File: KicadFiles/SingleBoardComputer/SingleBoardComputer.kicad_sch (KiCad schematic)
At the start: 83 parts, among them J1 USB_C_Receptacle_USB2.0_16P, J2 Conn_01x10_Pin, J3 Conn_01x06_Pin, J4 Conn_01x06_Pin, J5 Conn_01x06_Pin, SW1 SW_DPST_x2_Custom, U1 8468-11B1-RK-TP, U10 AS7C1026B-12JCN, U11 XC9572XL-PC44, U12 SST39SF040-70-4C-PHE, U13 SST39SF040-70-4C-PHE, U2 TLV809EA46DBZR, U3 TPS630701RNMT, U4 FT240XS, U5 LD1117S33TR_SOT223, U6 8444-11B1-RK-TP, U7 4832-6000-CP, U8 4832-6000-CP, U9 MC68000FN, Y1 CXO_DIP8

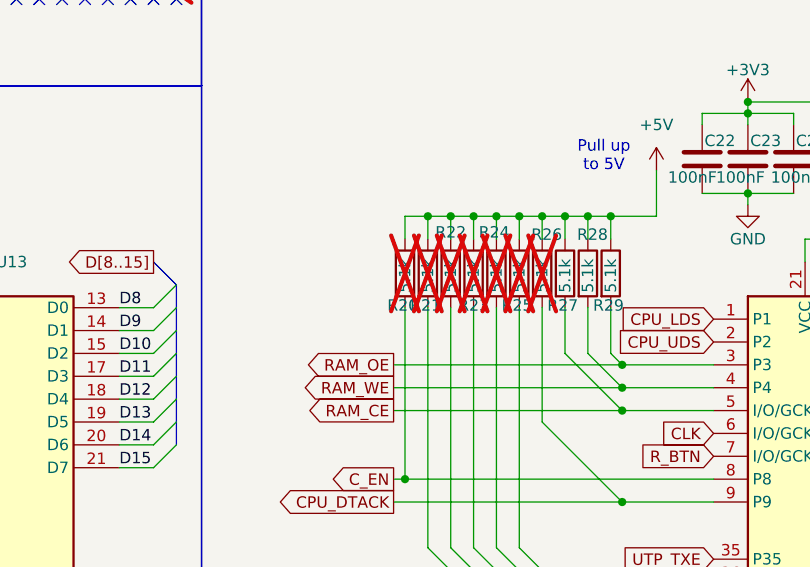
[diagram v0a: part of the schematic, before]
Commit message: PCB done
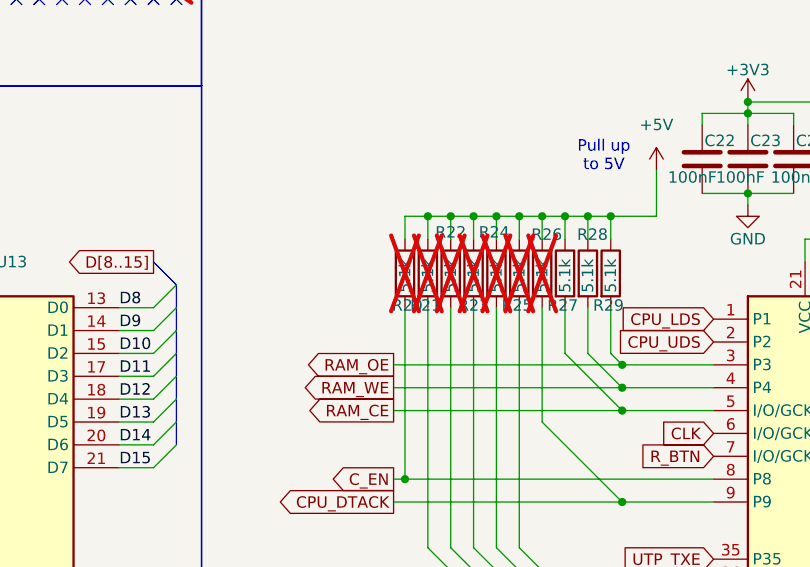
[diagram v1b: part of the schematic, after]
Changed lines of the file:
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@@
 			)
 		)
-		(property "Datasheet" "~"
+		(property "Datasheet" "https://www.digikey.com/en/products/detail/amphenol-cs-commercial-products/G800W302018EU/17069165"
 			(at 262.89 151.13 0)
 			(effects
@@
 			)
 		)
-		(property "Datasheet" "https://www.digikey.com/en/products/detail/adam-tech/PH1-10-UA/9830653?s=N4IgjCBcoGwJxVAYygMwIYBsDOBTANCAPZQDaIALGGABxwDsIAuoQA4AuUIAyuwE4BLAHYBzEAF9CNGohApIGHAWJkQMAMxwaMZm06Qe-YWMkg4ABlnzFeQiUjlNMGAFZdIDl16DREwmHh1KzQsWxUHEHUwODgAJgQWD31DHxN-egtghVDle3IGWJ1EzwNvYz9wLQRoORClO1VLJlNY81iIGuschoiqehoXBL0vI19TAFoZTrqwvJBWl0ZmwnGdach%2BAFdc1SDlkHHYrK2diLd98erkKBOe8ghm8XEgA"
+		(property "Datasheet" "https://www.digikey.com/en/products/detail/amphenol-cs-fci/10129378-910002BLF/7915958"
 			(at 180.34 105.41 0)
 			(effects
@@
 			)
 		)
-		(property "Datasheet" "https://www.digikey.com/en/products/detail/adam-tech/ADT-AMP1251106S4BS165A1/9832042"
+		(property "Datasheet" "https://www.digikey.com/en/products/detail/amphenol-cs-commercial-products/G800W302018EU/17069165"
 			(at 290.83 109.22 0)
 			(effects
@@
 		(lib_id "Device:R")
 		(at 208.28 191.77 0)
+		(mirror y)
 		(unit 1)
 		(exclude_from_sim no)
@@
 		(dnp yes)
 		(property "Reference" "R20"
-			(at 208.026 195.326 0)
+			(at 208.534 195.326 0)
 			(effects
 				(font
@@
 		)
 		(property "Footprint" "Resistor_SMD:R_0805_2012Metric_Pad1.20x1.40mm_HandSolder"
-			(at 206.502 191.77 90)
+			(at 210.058 191.77 90)
 			(effects
 				(font
@@
 			)
 		)
-		(property "Datasheet" "TPS630701RNMT"
+		(property "Datasheet" "https://www.digikey.com/en/products/detail/texas-instruments/TPS630701RNMT/6193742"
 			(at 148.59 48.26 0)
 			(effects
@@
 			)
 		)
-		(property "Datasheet" "~"
+		(property "Datasheet" "https://www.digikey.com/en/products/detail/amphenol-cs-commercial-products/G800W302018EU/17069165"
 			(at 224.79 151.13 0)
 			(effects
